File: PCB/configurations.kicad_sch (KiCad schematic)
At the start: 38 parts, among them J2 Conn_ARM_SWD_TagConnect_TC2030, J3 USB_C_Receptacle_USB2.0_16P, U1 XC7A50T-FGG484, U3 FT2232HQ, U4 M93C56-WMN6TP, U6 TPS62132, Y1 12MHz

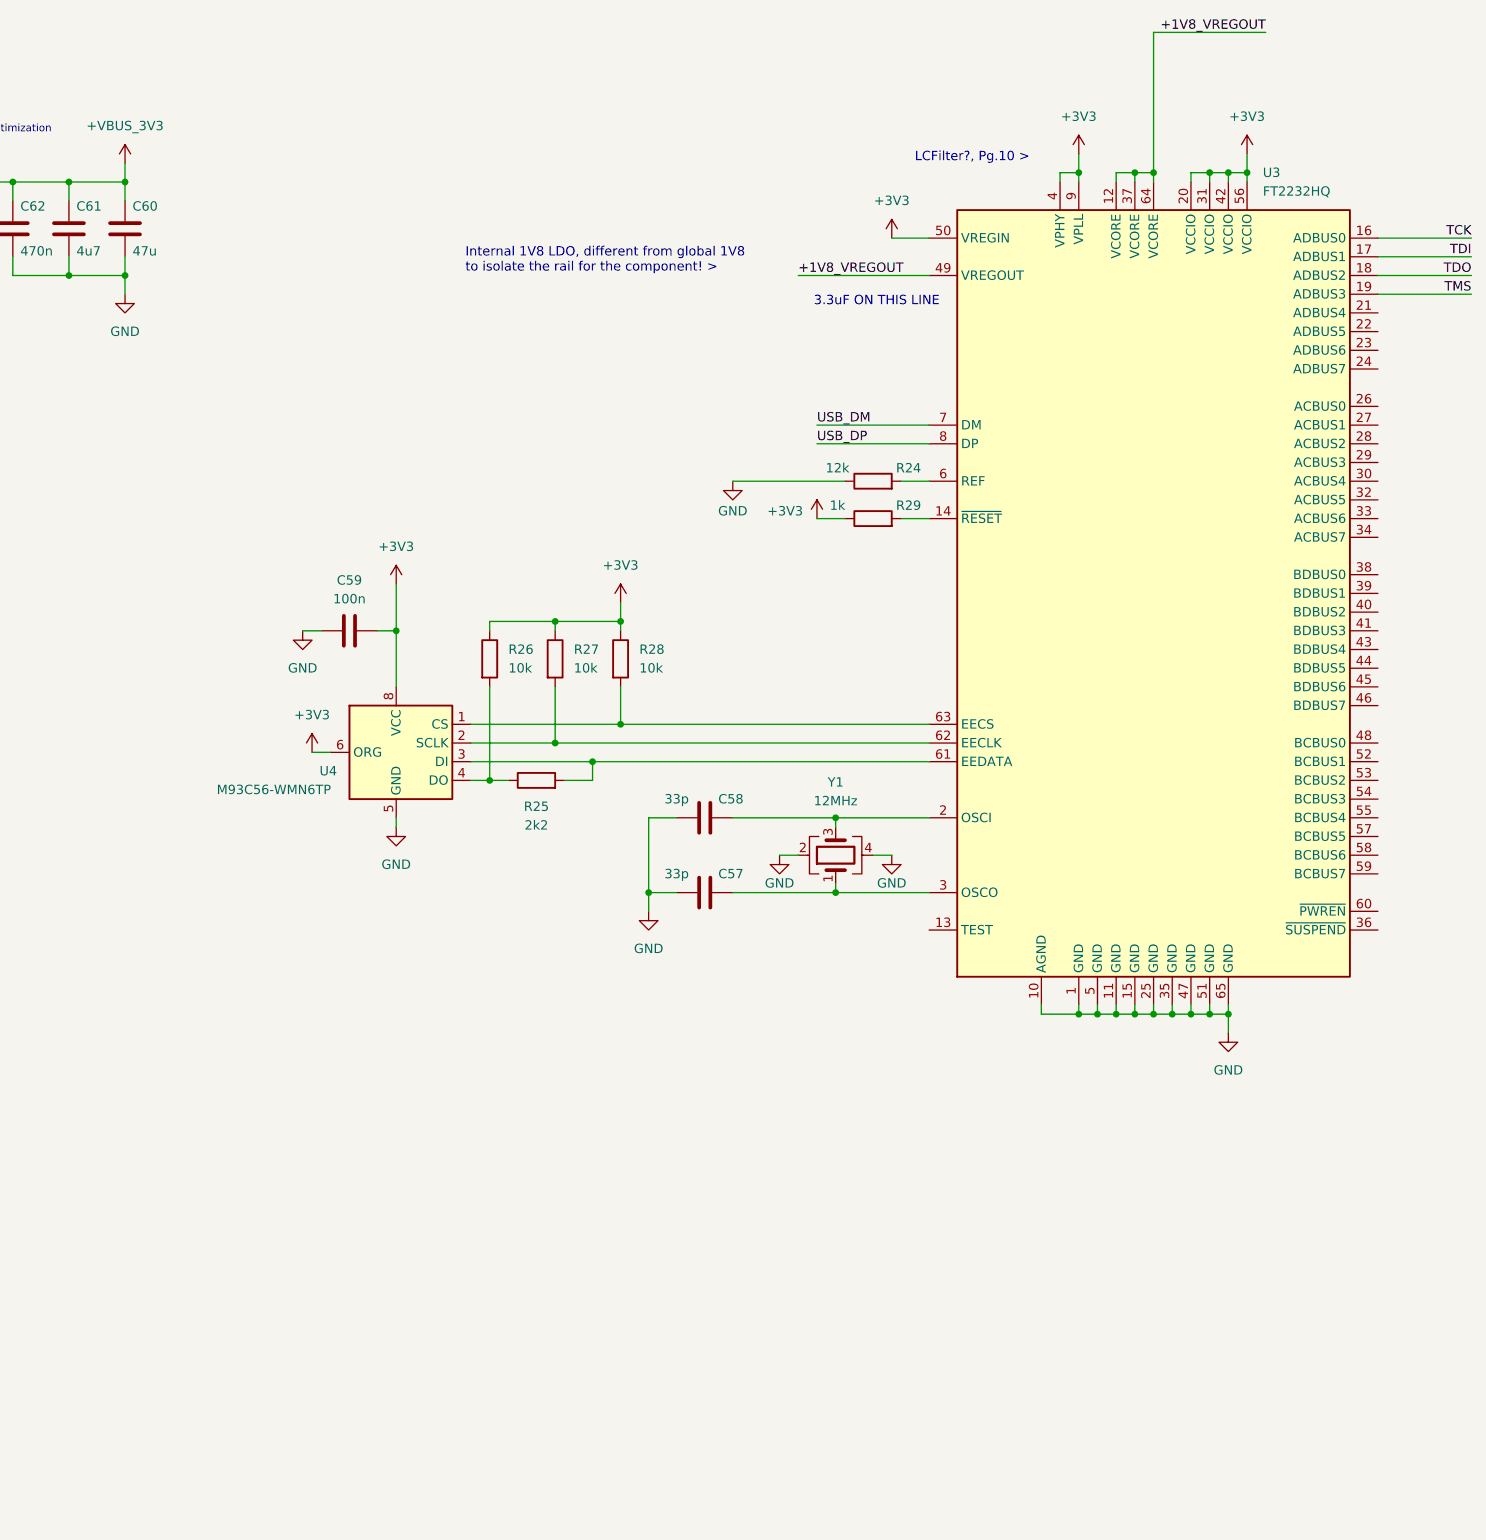
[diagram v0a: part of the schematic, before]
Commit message: decoupled all the rails
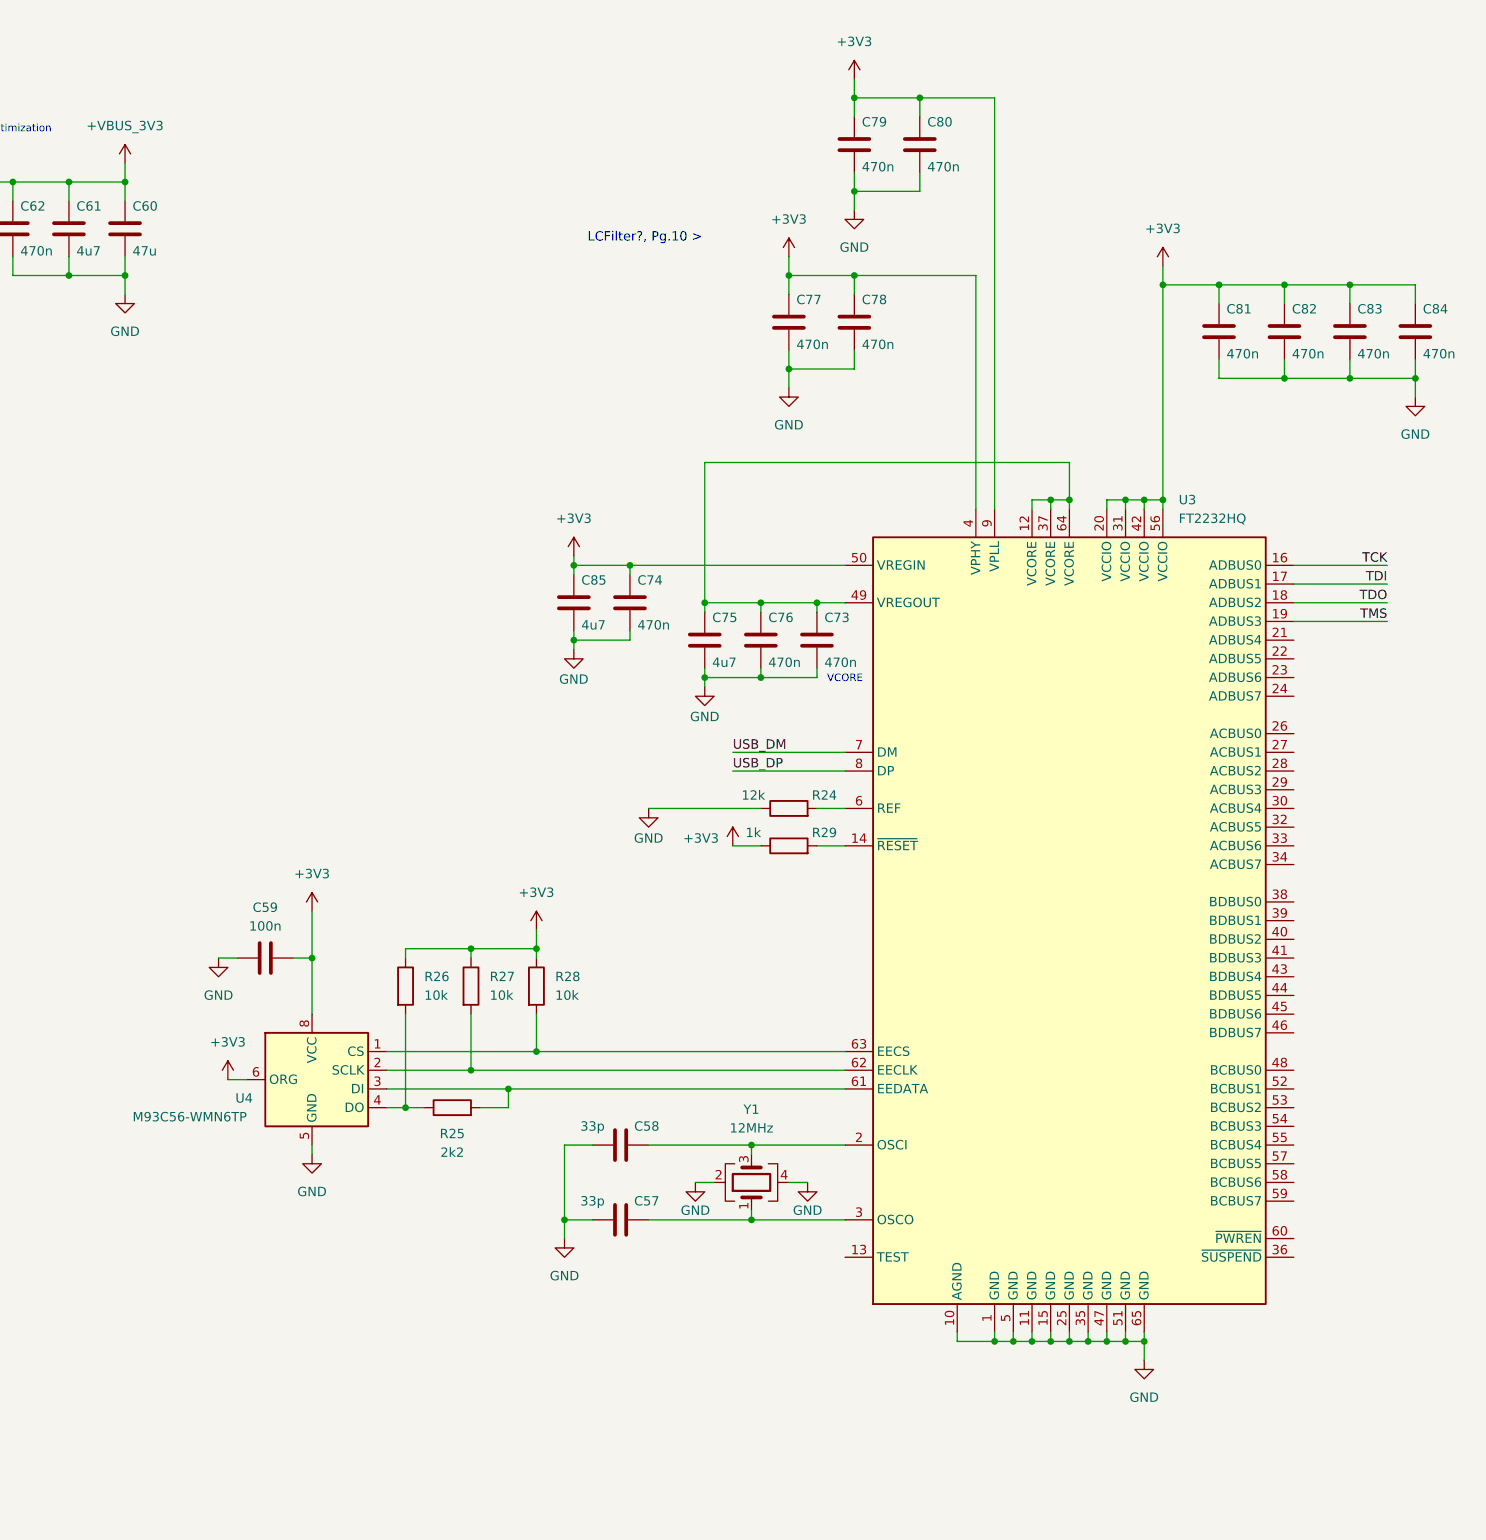
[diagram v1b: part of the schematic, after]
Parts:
- added C73, C74, C76, C77, C78, C79, C80, C81, C82, C83, C84: 470n, symbol Device:C
- added C75, C85: 4u7, symbol Device:C
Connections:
- net +3V3: now also C74.1, C77.1, C78.1, C79.1, C80.1, C81.1, C82.1, C83.1, C84.1, C85.1
- net GND: now also C73.2, C74.2, C75.2, C76.2, C77.2, C78.2, C79.2, C80.2, C81.2, C82.2, C83.2, C84.2, C85.2
- net +1V8_VREGOUT: no longer names the net of U3.12 (VCORE), U3.37 (VCORE), U3.49 (VREGOUT), U3.64 (VCORE)
- net +1V8_VREGOUT: now also C73.1, C75.1, C76.1
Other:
- note added: "VCORE"
- note removed: "3.3uF ON THIS LINE"
- note removed: "Internal 1V8 LDO, different from global 1V8 to isolate the rail for the component! >"
- moved on the sheet: C57, C58, C59, R24, R25, R26, R27, R28, R29, U3, U4, Y1
